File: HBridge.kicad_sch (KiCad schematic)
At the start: 20 parts

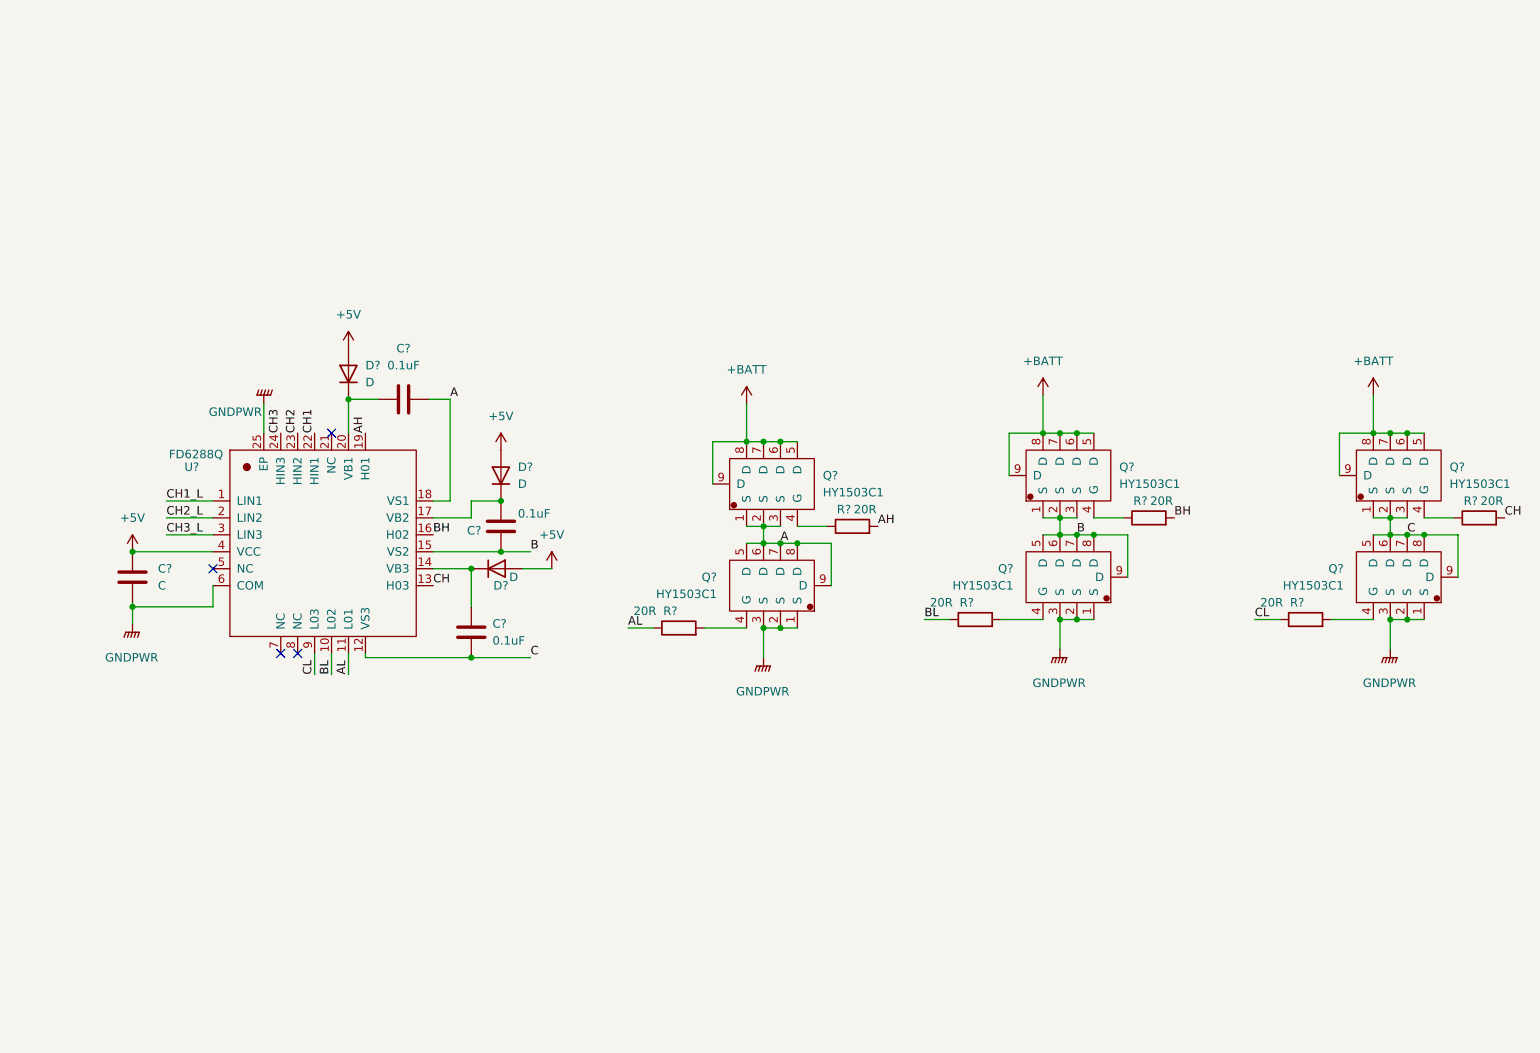
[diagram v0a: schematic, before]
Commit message: v0.9 finish
Signed-off-by: ncerzzk <huangzzk@bupt.edu.cn>
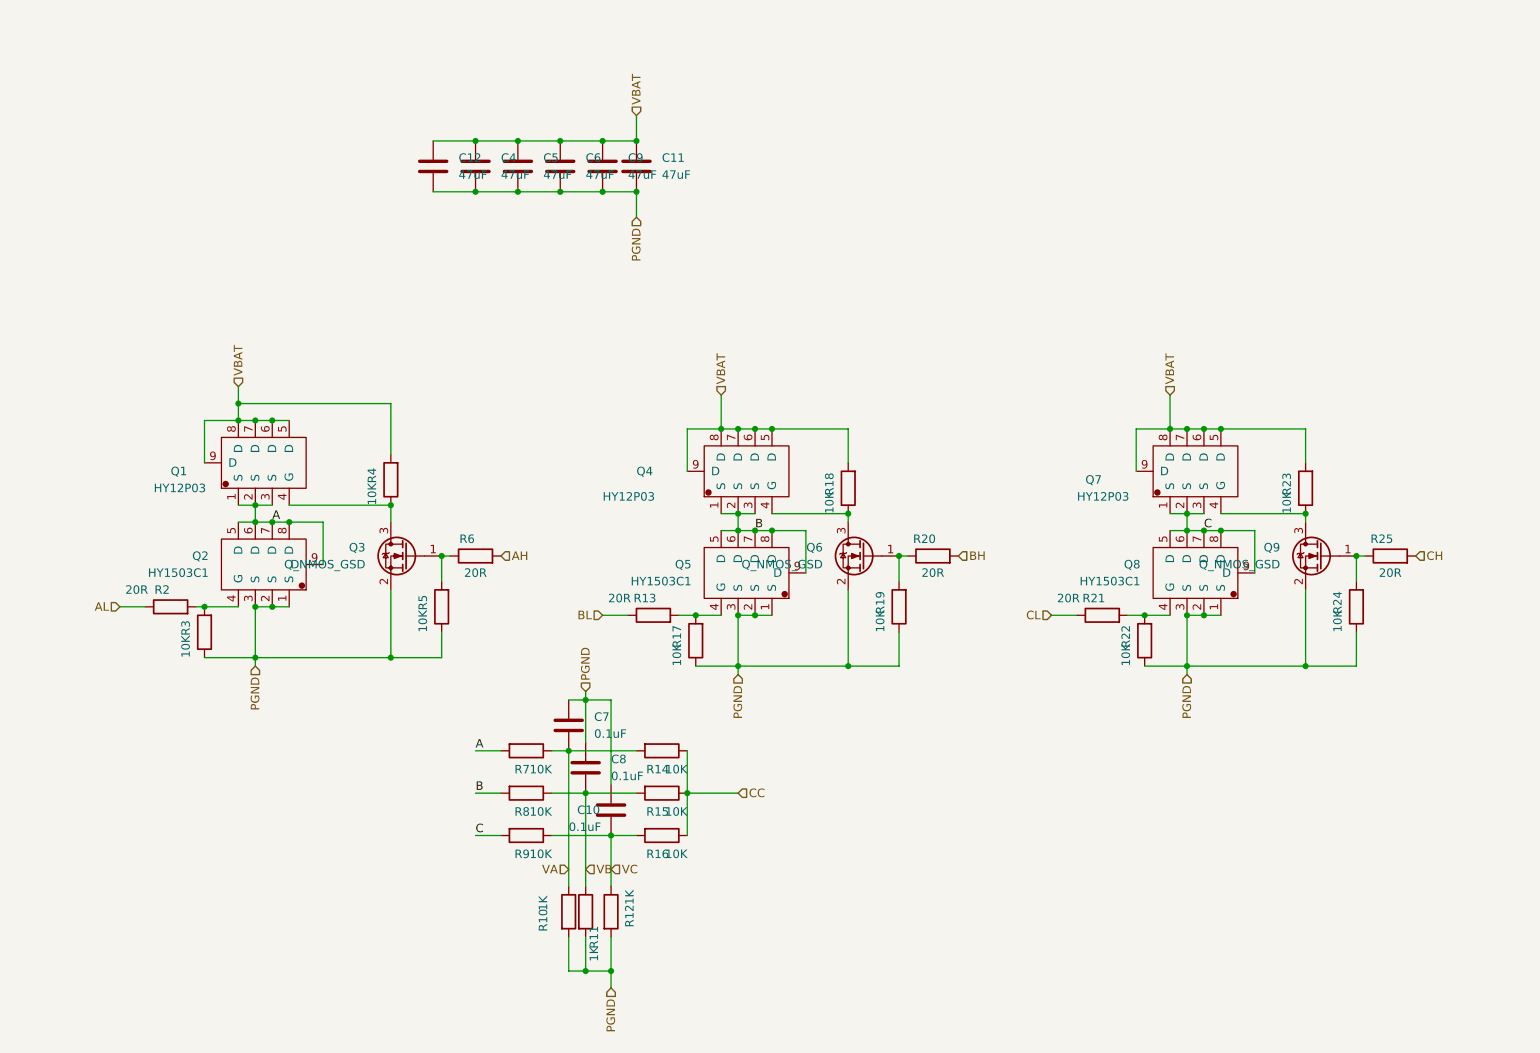
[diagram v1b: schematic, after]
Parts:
- removed C? (x3): 0.1uF, symbol Device:C
- removed C?: C, symbol Device:C
- removed D? (x3): D, symbol Device:D
- removed R? (x3): 20R, symbol Device:R
- removed U?: FD6288Q, Package_DFN_QFN:QFN-24-1EP_4x4mm_P0.5mm_EP2.65x2.65mm, symbol ic:FD6288Q
- added C10, C7, C8: 0.1uF, Capacitor_SMD:C_0402_1005Metric, symbol Device:C
- added C11, C12, C4, C5, C6, C9: 47uF, Capacitor_SMD:C_1206_3216Metric, symbol Device:C
- added Q3, Q6, Q9: Q_NMOS_GSD, Package_TO_SOT_SMD:SOT-23, symbol Device:Q_NMOS_GSD
- added R10, R11, R12: 1K, Resistor_SMD:R_0402_1005Metric, symbol Device:R
- added R14, R15, R16, R17, R18, R19, R22, R23, R24, R3, R4, R5, R7, R8, R9: 10K, Resistor_SMD:R_0402_1005Metric, symbol Device:R
- added R20, R25, R6: 20R, Resistor_SMD:R_0402_1005Metric, symbol Device:R
- Q1, Q4, Q7: renamed from Q?; value HY1503C1 -> HY12P03
- R13, R2, R21: renamed from R?; footprint (none) -> Resistor_SMD:R_0402_1005Metric
- gave numbers to parts that had none: 3
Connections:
- net A: now also R7.2
- net AH: now also R6.2
- net B: now also R8.2
- net BH: now also R20.2
- net C: now also R9.2
- net CH: now also R25.2
- net at Q1.4 (G): now also Q3.3 (D), R4.1
- net at Q5.4 (G), R13.2: now also R17.2
- net at Q8.4 (G), R21.2: now also R22.2
- net at Q4.4 (G): now also Q6.3 (D), R18.1
- net at Q7.4 (G): now also Q9.3 (D), R23.1
- net at Q2.4 (G), R2.2: now also R3.2
- net +BATT renamed VBAT
- net VBAT: now also C11.1, C12.1, C4.1, C5.1, C6.1, C9.1, R18.2, R23.2, R4.2
- net GNDPWR renamed PGND
- net PGND: now also C10.2, C11.2, C12.2, C4.2, C5.2, C6.2, C7.2, C8.2, C9.2, Q3.2 (S), Q6.2 (S), Q9.2 (S), R10.2, R11.2, R12.2, R17.1, R19.1, R22.1, R24.1, R3.1, R5.1
- new net: Q9.1 (G), R24.2, R25.1
- new net: Q3.1 (G), R5.2, R6.1
- new net: Q6.1 (G), R19.2, R20.1
- new net CC: R14.1, R15.1, R16.1
- new net VA: C7.1, R10.1, R14.2, R7.1
- new net VB: C8.1, R11.1, R15.2, R8.1
- new net VC: C10.1, R12.1, R16.2, R9.1
- no-connect marks 4 -> 0
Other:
- moved on the sheet: Q1, Q2, Q4, Q5, Q7, Q8, R13, R2, R21

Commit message: update for new version
Signed-off-by: huangzzk <huangcmzzk@gmail.com>
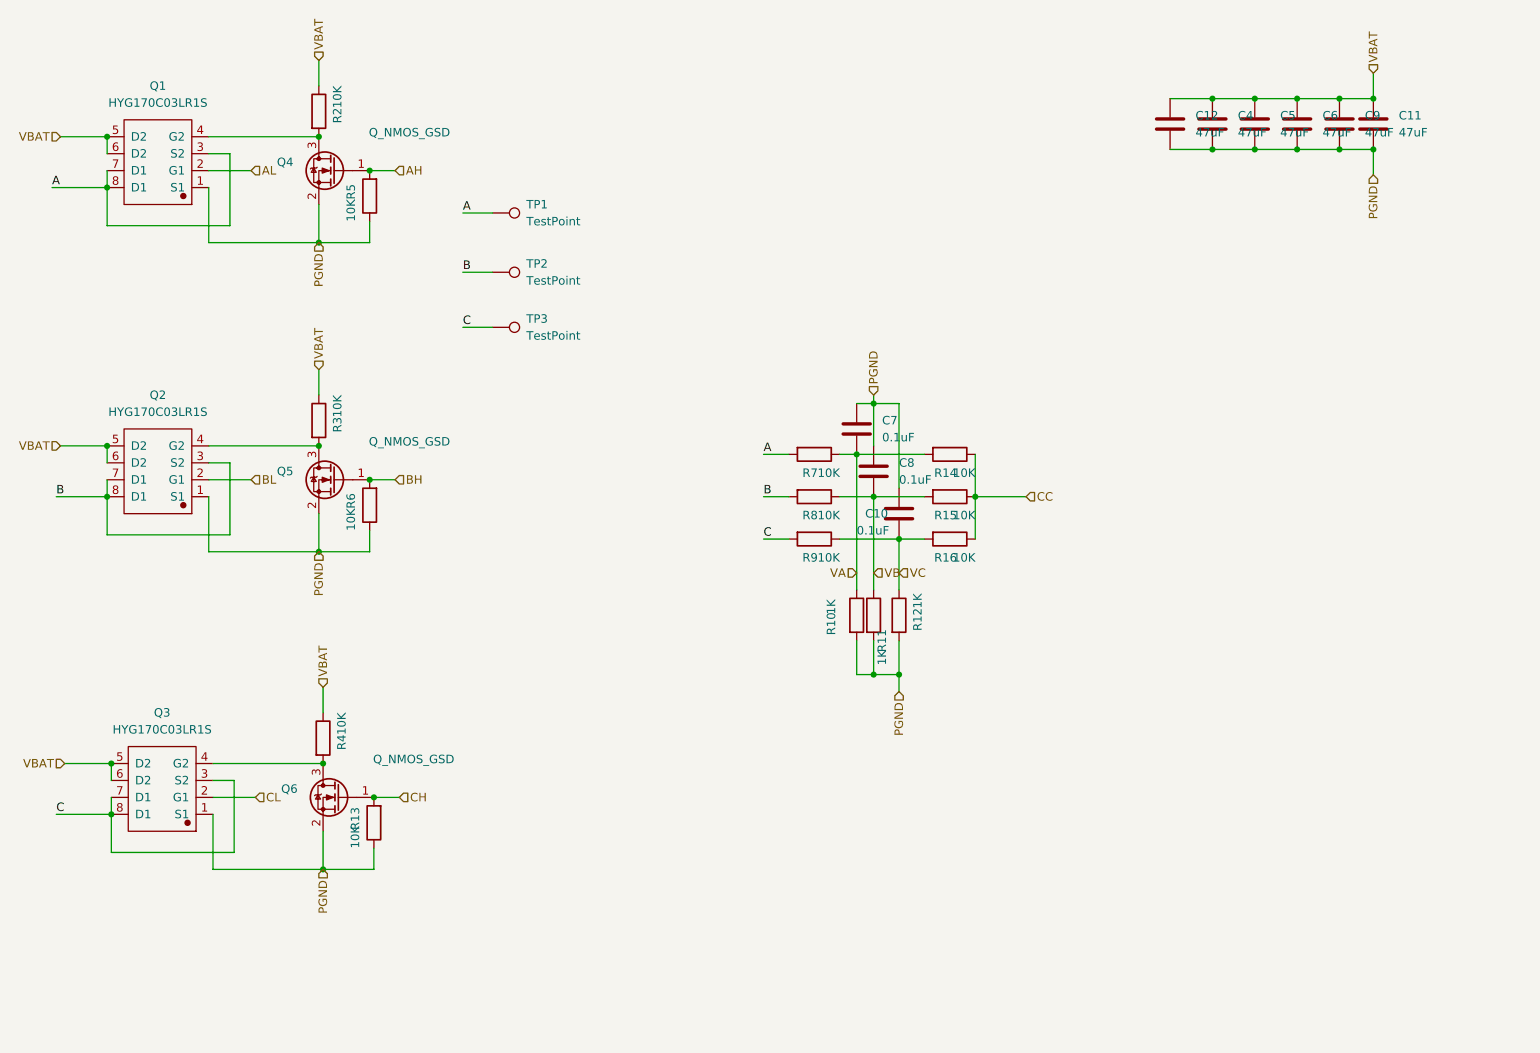
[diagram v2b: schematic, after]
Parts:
- removed Q1, Q4, Q7: HY12P03, Package_DFN_QFN:DFN-8-1EP_3x3mm_P0.65mm_EP1.7x2.05mm, symbol ic:HY1503C1
- removed Q2, Q5, Q8: HY1503C1, Package_DFN_QFN:DFN-8-1EP_3x3mm_P0.65mm_EP1.7x2.05mm, symbol ic:HY1503C1
- removed Q3, Q9: Q_NMOS_GSD, Package_TO_SOT_SMD:SOT-23, symbol Device:Q_NMOS_GSD
- removed R17, R18, R19, R22, R23, R24: 10K, Resistor_SMD:R_0402_1005Metric, symbol Device:R
- removed R20, R21, R25: 20R, Resistor_SMD:R_0402_1005Metric, symbol Device:R
- added Q1, Q2, Q3: HYG170C03LR1S, Package_SO:SO-8_3.9x4.9mm_P1.27mm, symbol ic:HYG170C03LR1S
- added Q4, Q5: Q_NMOS_GSD, Package_TO_SOT_SMD:SOT-23, symbol Device:Q_NMOS_GSD
- added TP1, TP2, TP3: TestPoint, TestPoint:TestPoint_THTPad_2.0x2.0mm_Drill1.0mm, symbol Connector:TestPoint
- R13, R2, R6: value 20R -> 10K
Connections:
- net A: now also Q1.3 (S2), Q1.7 (D1), Q1.8 (D1), TP1.1
- net AH: now also R5.2, Q4.1 (G); no longer R6.2
- net AL: now also Q1.2 (G1); no longer R2.1
- net B: now also Q2.3 (S2), Q2.7 (D1), Q2.8 (D1), TP2.1
- net BH: now also R6.2, Q5.1 (G)
- net BL: now also Q2.2 (G1); no longer R13.1
- net C: now also Q3.3 (S2), Q3.7 (D1), Q3.8 (D1), TP3.1
- net CH: now also Q6.1 (G), R13.2
- net CL: now also Q3.2 (G1)
- net PGND: now also R13.1, R6.1, Q1.1 (S1), Q2.1 (S1), Q3.1 (S1), Q4.2 (S), Q5.2 (S); no longer R3.1
- net VBAT: now also R2.1, R3.1, R4.1, Q1.5 (D2), Q1.6 (D2), Q2.5 (D2), Q2.6 (D2), Q3.5 (D2), Q3.6 (D2); no longer R4.2
- net at Q6.3 (D): now also R4.2, Q3.4 (G2)
- net at R2.2: now also Q1.4 (G2), Q4.3 (D); no longer R3.2
- new net: Q2.4 (G2), Q5.3 (D), R3.2
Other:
- moved on the sheet: C10, C11, C12, C4, C5, C6, C7, C8, C9, R10, R11, R12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
